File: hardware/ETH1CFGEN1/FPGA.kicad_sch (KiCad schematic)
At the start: 45 parts, among them J202 Conn_02x07_Odd_Even, U201 TLV1117LV33DCYR, U202 TLV1117LV12DCYR, U203 XC6SLX9-3TQG144I, U204 W25Q64JV, X201 ASFL1-100.000MHZ-L-T

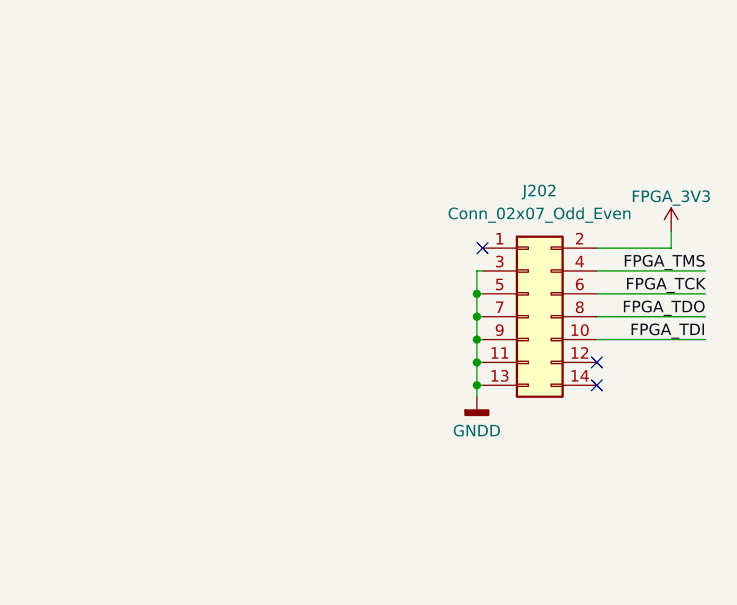
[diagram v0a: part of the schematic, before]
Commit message: PCB design
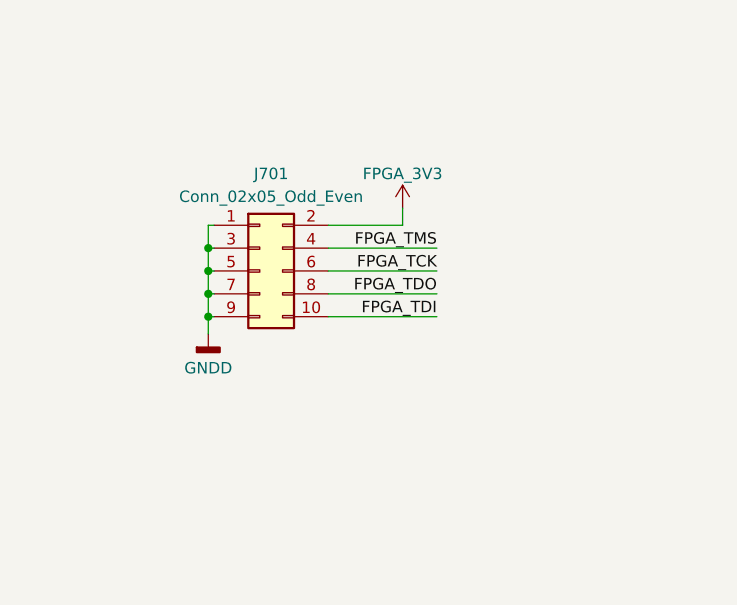
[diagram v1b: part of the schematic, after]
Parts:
- removed J202: Conn_02x07_Odd_Even, symbol Connector_Generic:Conn_02x07_Odd_Even
- added J701: Conn_02x05_Odd_Even, Connector_PinHeader_2.54mm:PinHeader_2x05_P2.54mm_Vertical, symbol Connector_Generic:Conn_02x05_Odd_Even
- X201: footprint (none) -> Crystal:Crystal_SMD_5032-4Pin_5.0x3.2mm
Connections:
- net FPGA_3V3: now also J701.2 (Pin_2)
- net FPGA_TCK: now also J701.6 (Pin_6)
- net FPGA_TDI: now also J701.10 (Pin_10)
- net FPGA_TDO: now also J701.8 (Pin_8)
- net FPGA_TMS: now also J701.4 (Pin_4)
- net GNDD: now also J701.1 (Pin_1), J701.3 (Pin_3), J701.5 (Pin_5), J701.7 (Pin_7), J701.9 (Pin_9)
- no-connect marks 3 -> 0
